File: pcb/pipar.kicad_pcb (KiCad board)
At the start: 2 copper layers, 139.4 x 159.1 mm, 133 parts, among them M2 MountingHole_2.2mm_M2, SW1 SW_Wuerth_450301014042, SW2 SW_Wuerth_450301014042, U2 nice_nano

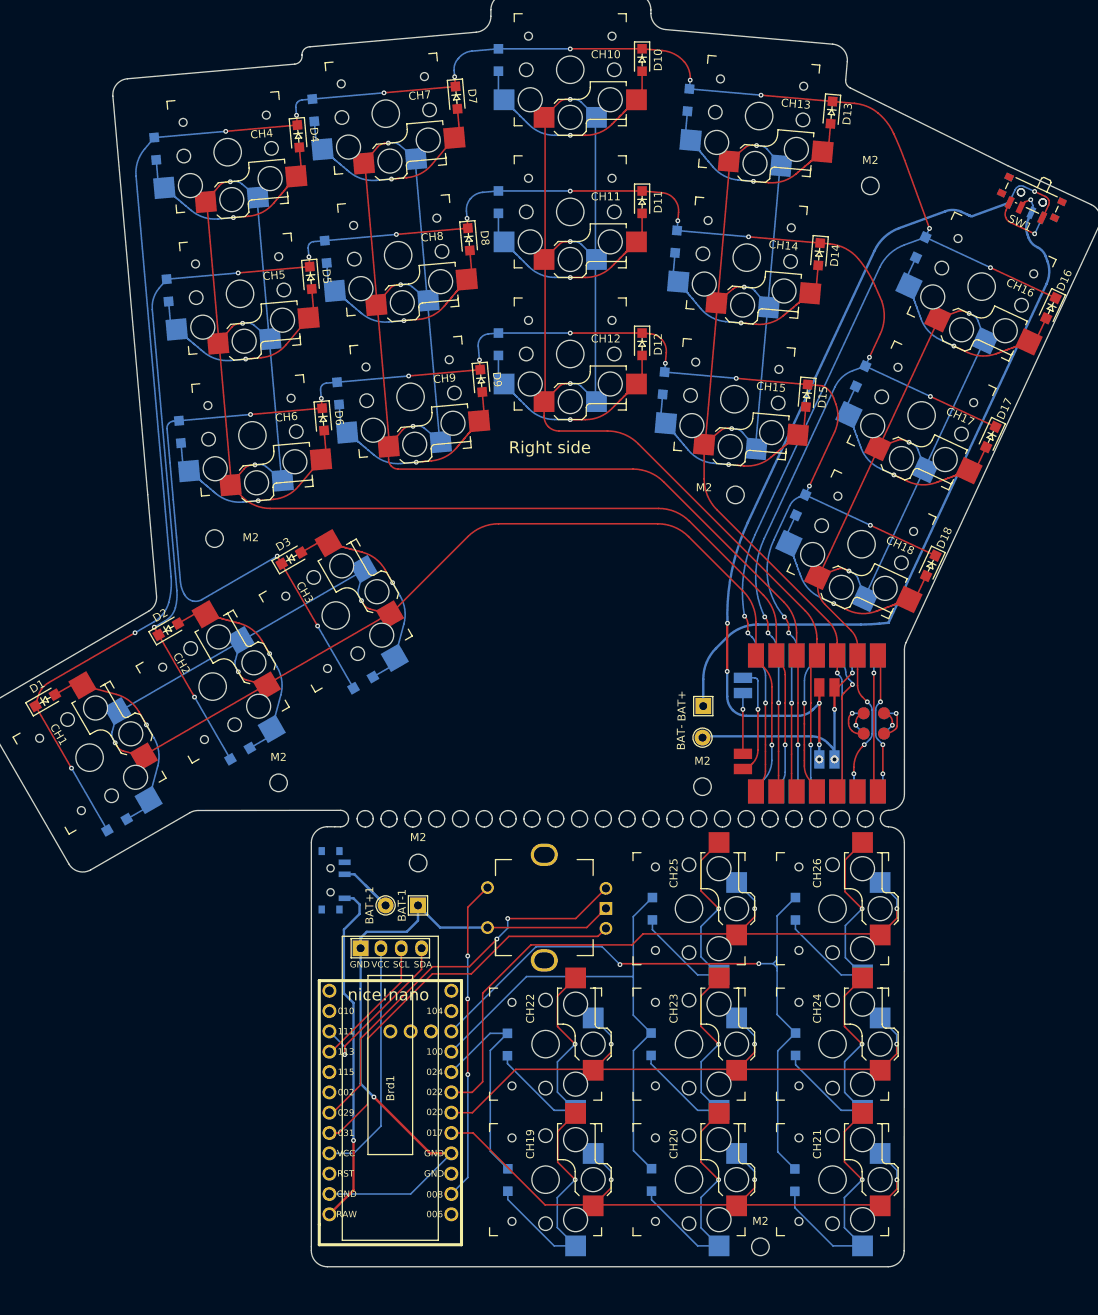
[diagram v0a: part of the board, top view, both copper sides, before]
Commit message: Improved schematics and PCBs
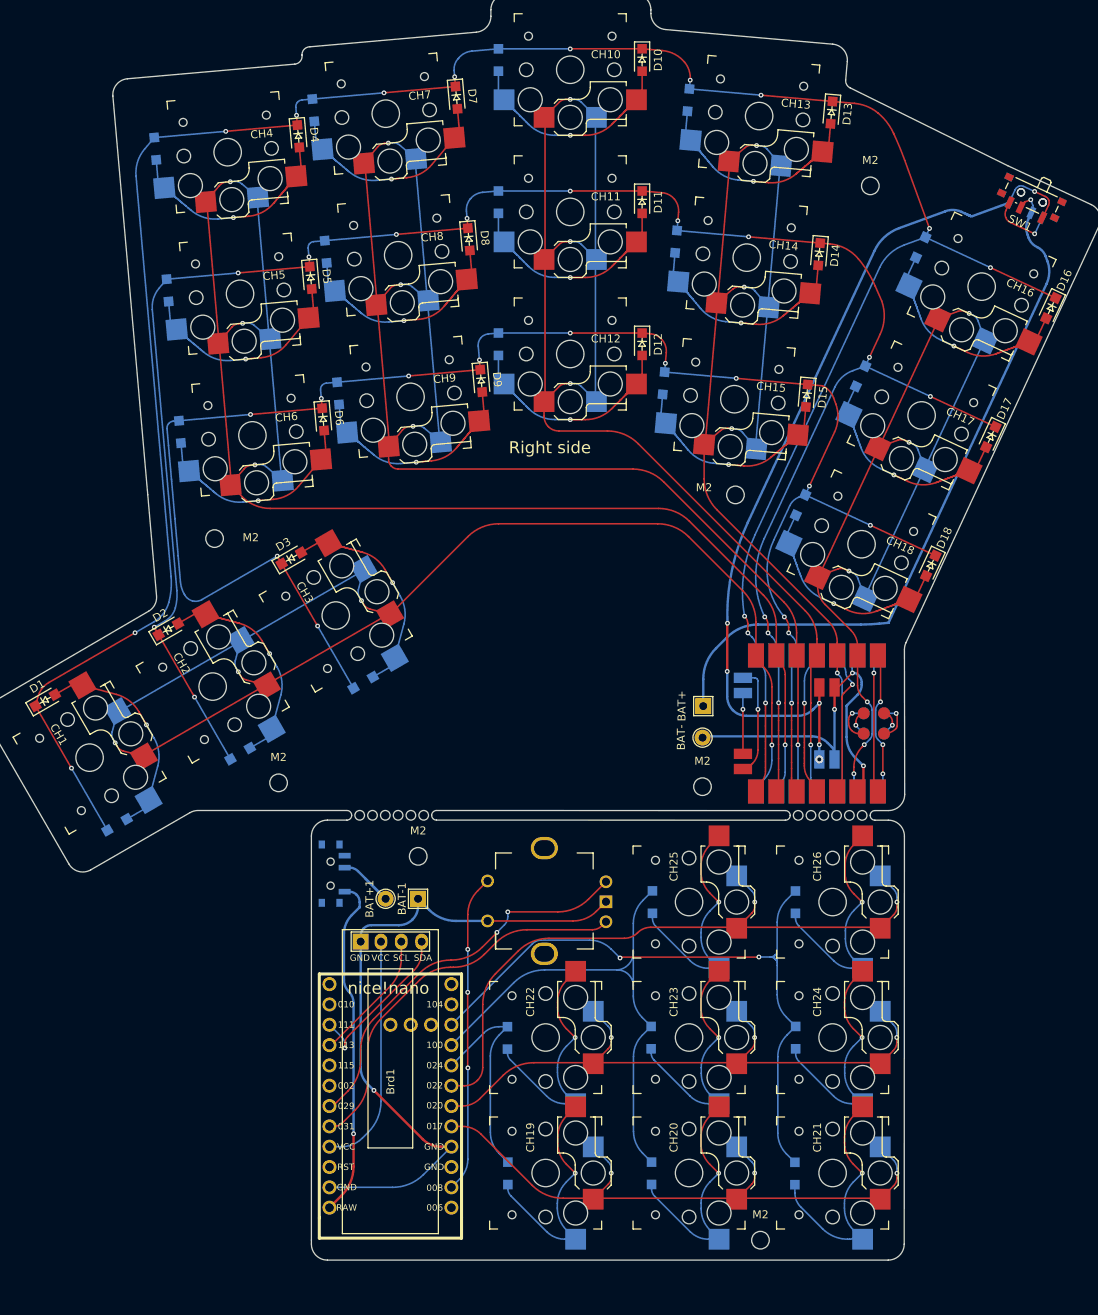
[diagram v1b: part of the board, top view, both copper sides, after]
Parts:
- removed CH27: RotaryEncoder_Switch, Rotary_Encoder:RotaryEncoder_Bourns_Vertical_PEL11L-4xxxF-Sxxxx_1
- added CH28: RotaryEncoder_Switch, Rotary_Encoder:RotaryEncoder_Bourns_Vertical_PEL11L-4xxxF-Sxxxx_1, F.Cu at (82.6, 130.3)
- moved BAT+1 0.83 mm to (62.8, 129.9)
- moved BAT-1 0.83 mm to (66.9, 129.9)
- moved Brd1 0.83 mm to (63.5, 152.8)
- moved CH19 0.83 mm to (82.8, 164.2)
- moved CH20 0.83 mm to (100.8, 164.2)
- moved CH21 0.83 mm to (118.7, 164.2)
- moved CH22 0.83 mm to (82.8, 147.3)
- moved CH23 0.83 mm to (100.8, 147.3)
- moved CH24 0.83 mm to (118.7, 147.3)
- moved CH25 0.83 mm to (100.8, 130.4)
- moved D19 0.83 mm to (78.1, 164.3)
- moved D20 0.83 mm to (96.1, 164.3)
- moved D21 0.83 mm to (114.0, 164.3)
- moved SW2 0.83 mm to (56.3, 126.8)
- moved M2 0.83 mm to (66.9, 124.6)
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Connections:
- U2 pad 3: unconnected-(U2-GND-Pad3) -> GND
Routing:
- net GND: track 119.0 -> 134.8 mm
- net Net-(D20-K): track 64.3 -> 67.7 mm
- net Net-(D21-A): track 32.8 -> 30.0 mm
- net Net-(D19-A): track 32.2 -> 29.8 mm
- net Net-(D23-A): track 32.2 -> 29.8 mm
- net Net-(D22-A): track 32.2 -> 29.8 mm
- net Net-(D26-A): track 32.0 -> 29.6 mm
- net Net-(U2-P0.22): track 85.5 -> 84.0 mm
- net Net-(U2-AIN7/P0.31): track 50.0 -> 48.5 mm
- net Net-(U2-AIN5/P0.29): track 50.3 -> 48.9 mm
- net Net-(U2-P0.17): track 83.4 -> 82.3 mm
- net Net-(U2-P0.20): track 81.9 -> 80.8 mm
- net Net-(D25-A): track 32.2 -> 31.2 mm
- net Net-(D24-A): track 32.1 -> 31.2 mm
- net Net-(D20-A): track 32.2 -> 31.2 mm
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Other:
- board size 139.4 x 159.1 mm -> 139.4 x 158.3 mm

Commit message: updates pcb and zmk, forgot to use i2c pins
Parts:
- added U1: Seeeduino Xiao nRF52840, Seeed Studio XIAO Series Library:XIAO-nRF52840-Sense-14P-2.54-21X17.8MM, F.Cu at (198.8, -32.5)
- moved D4 180.0 mm to (208.4, -8.69), turned to -175 degrees
- moved D1 174.6 mm to (139.4, -22.4), turned to -60 degrees
- moved CH4 168.8 mm to (207.9, 0.36), turned to -85 degrees
- moved CH1 167.4 mm to (132.3, -16.9), turned to 30 degrees
- moved D5 166.7 mm to (190.7, -7.14), turned to -175 degrees
- moved D1 164.2 mm to (123.9, -13.5), turned to -60 degrees
- moved D7 160.7 mm to (213.2, 11.1), turned to -175 degrees
- moved D4 160.0 mm to (209.9, 9.20), turned to -175 degrees
- moved D6 156.2 mm to (173.0, -5.60), turned to -175 degrees
- moved CH5 154.7 mm to (190.2, 1.91), turned to -85 degrees
- moved D2 152.8 mm to (148.3, -7.06), turned to -60 degrees
- moved CH7 150.3 mm to (212.8, 20.1), turned to -85 degrees
- moved M2 146.3 mm to (159.6, -1.28), turned to -90 degrees
- moved CH2 144.9 mm to (141.1, -1.51), turned to 30 degrees
- moved D5 144.8 mm to (192.2, 10.7), turned to -175 degrees
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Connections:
- CH19 pad 1: Net-(U2-P0.17) -> Net-(U2-P1.15)
- CH20 pad 1: Net-(U2-P0.17) -> Net-(U2-P1.15)
- CH21 pad 1: Net-(U2-P0.17) -> Net-(U2-P1.15)
- CH22 pad 1: Net-(U2-P0.20) -> Net-(U2-P1.13)
- CH23 pad 1: Net-(U2-P0.20) -> Net-(U2-P1.13)
- CH24 pad 1: Net-(U2-P0.20) -> Net-(U2-P1.13)
- CH25 pad 1: Net-(U2-P0.22) -> Net-(U2-P1.11)
- CH26 pad 1: Net-(U2-P0.22) -> Net-(U2-P1.11)
- U2 pad 15: Net-(Brd1-SDA) -> Net-(U2-P1.11)
- U2 pad 16: Net-(Brd1-SCL) -> Net-(U2-P1.13)
- U2 pad 17: unconnected-(U2-P1.15-Pad17) -> Net-(U2-P1.15)
- U2 pad 5: Net-(U2-P0.17) -> Net-(Brd1-SDA)
- U2 pad 6: Net-(U2-P0.20) -> Net-(Brd1-SCL)
- U2 pad 7: Net-(U2-P0.22) -> unconnected-(U2-P0.22-Pad7)
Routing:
- net Net-(U2-P1.15): track 0.00 -> 118.7 mm, vias 0 -> 6
- net Net-(U2-P1.13): track 0.00 -> 100.6 mm, vias 0 -> 4
- net Net-(U2-P1.11): track 0.00 -> 90.8 mm, vias 0 -> 2
- net Net-(U2-P0.22): track 84.0 -> 0.00 mm, vias 2 -> 0
- net Net-(U2-P0.17): track 82.3 -> 0.00 mm, vias 3 -> 0
- net Net-(U2-P0.20): track 80.8 -> 0.00 mm, vias 3 -> 0
- net Net-(U2-AIN5/P0.29): track 48.9 -> 62.8 mm, vias 2 -> 1
- net Net-(U2-AIN7/P0.31): track 48.5 -> 60.5 mm, vias 0 -> 1
- net Net-(D20-K): track 67.7 -> 60.3 mm, vias 0 -> 1
- net Net-(Brd1-SCL): track 16.5 -> 23.9 mm, vias 0 -> 1
- net Net-(Brd1-SDA): track 20.7 -> 24.6 mm, vias 1 -> 0
- net Net-(U2-RX1/P0.08): track 39.8 -> 43.6 mm, vias 3 -> 0
- net Net-(D19-K): track 27.3 -> 23.5 mm, vias 0 -> 1
- net Net-(SW2-C): track 10.3 -> 6.73 mm
- net GND: track 134.8 -> 137.1 mm, vias 4 -> 3
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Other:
- board size 139.4 x 158.3 mm -> 158.3 x 139.4 mm
